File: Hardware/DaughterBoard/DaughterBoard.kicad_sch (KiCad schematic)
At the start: 19 parts, among them J1 CARTDRIGE, J10 JOYPAD2, J11 LCD, J12 POWER, J13 PA, J14 PB, J2 ROM, J3 ISA00, J4 ISA10, J7 ISA01, J8 ISA11, J9 JOYPAD1, X1 ACO-20MHz

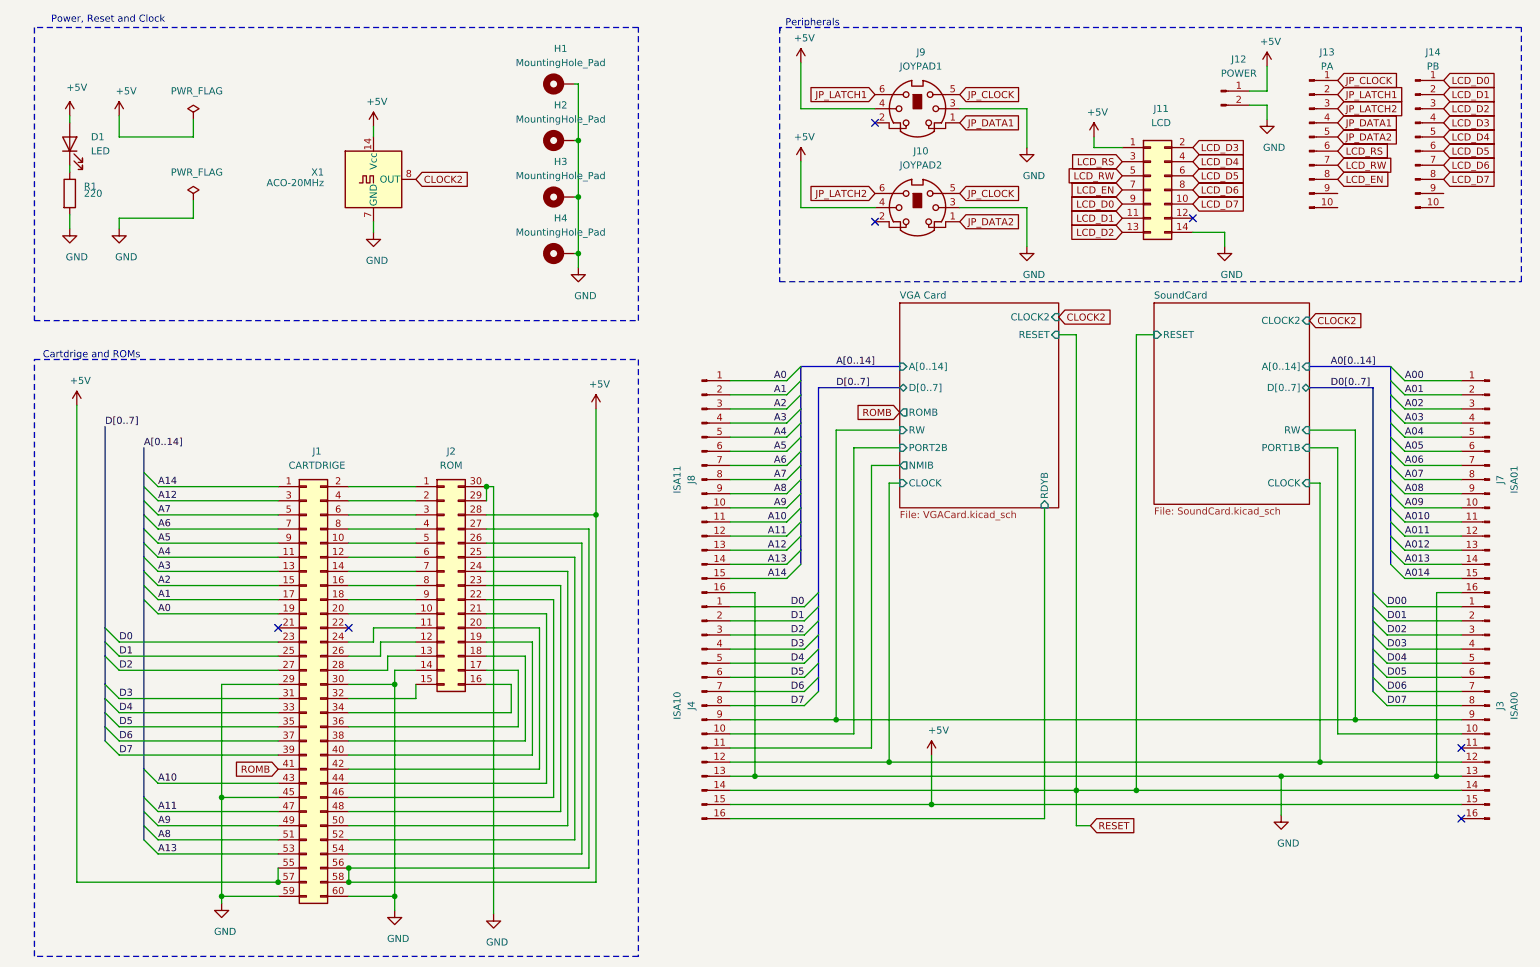
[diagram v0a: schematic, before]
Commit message: Version 1.2
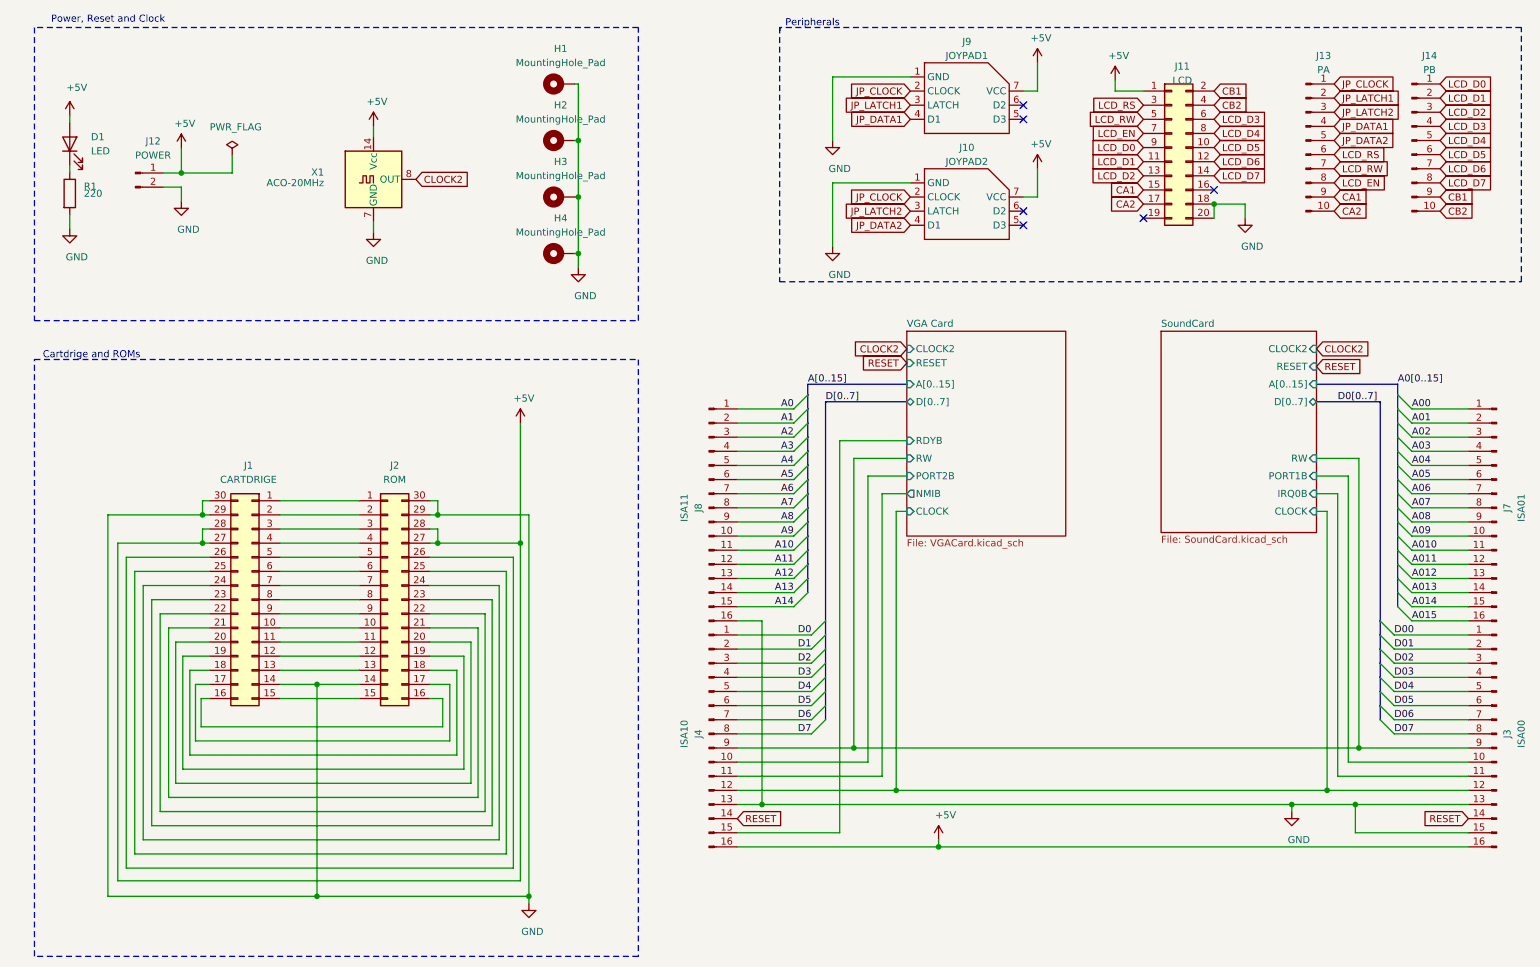
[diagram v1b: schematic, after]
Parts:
- removed J10: JOYPAD2, Connector_PinSocket_2.54mm:PinSocket_2x04_P2.54mm_Vertical, symbol Connector:Mini-DIN-6
- removed J9: JOYPAD1, Connector_PinSocket_2.54mm:PinSocket_2x04_P2.54mm_Vertical, symbol Connector:Mini-DIN-6
- added J10: JOYPAD2, Connector_TheRLab:NES_JoyPad, symbol Connector_TheRLab:NES_JoyPad
- added J9: JOYPAD1, Connector_TheRLab:NES_JoyPad, symbol Connector_TheRLab:NES_JoyPad
- J1: footprint Connector_PinSocket_2.54mm:PinSocket_2x30_P2.54mm_Vertical -> Connector_PinHeader_2.54mm:PinHeader_2x15_P2.54mm_Vertical; symbol Connector_Generic:Conn_02x30_Odd_Even -> Connector_Generic:Conn_02x15_Counter_Clockwise
- J11: footprint Connector_PinHeader_2.54mm:PinHeader_2x07_P2.54mm_Vertical -> Connector_IDC:IDC-Header_2x10_P2.54mm_Vertical; symbol Connector_Generic:Conn_02x07_Odd_Even -> Connector_Generic:Conn_02x10_Odd_Even
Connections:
- net +5V: now also J1.27 (Pin_27), J1.28 (Pin_28), J3.16 (Pin_16), J4.16 (Pin_16), J10.7 (VCC), J9.7 (VCC); no longer J1.55 (Pin_55), J1.56 (Pin_56), J1.57 (Pin_57), J1.58 (Pin_58), J3.15 (Pin_15), J4.15 (Pin_15)
- net A0: no longer J1.19 (Pin_19)
- net A1: no longer J1.17 (Pin_17)
- net A10: no longer J1.43 (Pin_43)
- net A11: no longer J1.47 (Pin_47)
- net A12: no longer J1.3 (Pin_3)
- net A13: no longer J1.53 (Pin_53)
- net A14: no longer J1.1 (Pin_1)
- net A2: no longer J1.15 (Pin_15)
- net A3: no longer J1.13 (Pin_13)
- net A4: no longer J1.11 (Pin_11)
- net A5: no longer J1.9 (Pin_9)
- net A6: no longer J1.7 (Pin_7)
- net A7: no longer J1.5 (Pin_5)
- net A8: no longer J1.51 (Pin_51)
- net A9: no longer J1.49 (Pin_49)
- net D0: no longer J1.23 (Pin_23)
- net D1: no longer J1.25 (Pin_25)
- net D2: no longer J1.27 (Pin_27)
- net D3: no longer J1.31 (Pin_31)
- net D4: no longer J1.33 (Pin_33)
- net D5: no longer J1.35 (Pin_35)
- net D6: no longer J1.37 (Pin_37)
- net D7: no longer J1.39 (Pin_39)
- net GND: now also J1.14 (Pin_14), J11.18 (Pin_18), J11.20 (Pin_20), J3.15 (Pin_15), J10.1 (GND), J9.1 (GND); no longer J1.45 (Pin_45), J1.59 (Pin_59), J1.60 (Pin_60), J11.14 (Pin_14), J7.16 (Pin_16)
- net JP_CLOCK: now also J10.2 (CLOCK), J9.2 (CLOCK)
- net JP_DATA1: now also J9.4 (D1)
- net JP_DATA2: now also J10.4 (D1)
- net JP_LATCH1: now also J9.3 (LATCH)
- net JP_LATCH2: now also J10.3 (LATCH)
- net LCD_D3: now also J11.6 (Pin_6); no longer J11.2 (Pin_2)
- net LCD_D4: now also J11.8 (Pin_8); no longer J11.4 (Pin_4)
- net LCD_D5: now also J11.10 (Pin_10); no longer J11.6 (Pin_6)
- net LCD_D6: now also J11.12 (Pin_12); no longer J11.8 (Pin_8)
- net LCD_D7: now also J11.14 (Pin_14); no longer J11.10 (Pin_10)
- net VGA Card/RDYB: now also J4.15 (Pin_15); no longer J4.16 (Pin_16)
- net at J2.1 (Pin_1): now also J1.1 (Pin_1); no longer J1.2 (Pin_2)
- net at J2.10 (Pin_10): now also J1.10 (Pin_10); no longer J1.20 (Pin_20)
- net at J2.11 (Pin_11): now also J1.11 (Pin_11); no longer J1.24 (Pin_24)
- net at J2.12 (Pin_12): now also J1.12 (Pin_12); no longer J1.26 (Pin_26)
- net at J2.13 (Pin_13): now also J1.13 (Pin_13); no longer J1.28 (Pin_28)
- net at J2.15 (Pin_15): now also J1.15 (Pin_15); no longer J1.32 (Pin_32)
- net at J2.16 (Pin_16): now also J1.16 (Pin_16); no longer J1.34 (Pin_34)
- net at J2.17 (Pin_17): now also J1.17 (Pin_17); no longer J1.36 (Pin_36)
- net at J2.18 (Pin_18): now also J1.18 (Pin_18); no longer J1.38 (Pin_38)
- net at J2.19 (Pin_19): now also J1.19 (Pin_19); no longer J1.40 (Pin_40)
- net at J2.2 (Pin_2): now also J1.2 (Pin_2); no longer J1.4 (Pin_4)
- net at J2.20 (Pin_20): now also J1.20 (Pin_20); no longer J1.42 (Pin_42)
- net at J2.21 (Pin_21): now also J1.21 (Pin_21); no longer J1.44 (Pin_44)
- net at J2.22 (Pin_22): now also J1.22 (Pin_22); no longer J1.46 (Pin_46)
- net at J2.23 (Pin_23): now also J1.23 (Pin_23); no longer J1.48 (Pin_48)
- net at J2.24 (Pin_24): now also J1.24 (Pin_24); no longer J1.50 (Pin_50)
- net at J2.25 (Pin_25): now also J1.25 (Pin_25); no longer J1.52 (Pin_52)
- net at J2.26 (Pin_26): now also J1.26 (Pin_26); no longer J1.54 (Pin_54)
- net at J2.3 (Pin_3): now also J1.3 (Pin_3); no longer J1.6 (Pin_6)
- net at J2.4 (Pin_4): now also J1.4 (Pin_4); no longer J1.8 (Pin_8)
- net at J2.5 (Pin_5): now also J1.5 (Pin_5); no longer J1.10 (Pin_10)
- net at J2.6 (Pin_6): now also J1.6 (Pin_6); no longer J1.12 (Pin_12)
- net at J2.7 (Pin_7): now also J1.7 (Pin_7); no longer J1.14 (Pin_14)
- net at J2.8 (Pin_8): now also J1.8 (Pin_8); no longer J1.16 (Pin_16)
- net at J2.9 (Pin_9): now also J1.9 (Pin_9); no longer J1.18 (Pin_18)
- net SoundCard/IRQ0B: now reaches J3.11 (Pin_11)
- net CA2: now reaches J13.10 (Pin_10)
- net CA2: now also J11.17 (Pin_17)
- net CA1: now reaches J13.9 (Pin_9)
- net CA1: now also J11.15 (Pin_15)
- net CB2: now reaches J14.10 (Pin_10)
- net CB2: now also J11.4 (Pin_4)
- net CB1: now reaches J14.9 (Pin_9)
- net CB1: now also J11.2 (Pin_2)
- removed net ROMB: J1.41 (Pin_41)
- new net A015: J7.16 (Pin_16)
- no-connect marks 7 -> 6
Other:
- sheet SoundCard ports: added A[0..15], IRQ0B; removed A[0..14]
- sheet VGA Card ports: added A[0..15]; removed A[0..14], ROMB
- moved on the sheet: J12, J13, J14, J2, J3, J4, J7, J8
